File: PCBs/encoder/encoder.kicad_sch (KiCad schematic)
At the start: 16 parts, among them J1 Conn_01x04, J2 Conn_01x04, J3 Conn_01x04, U1 AS5600-ASOT, U2 STM32G031G6Ux

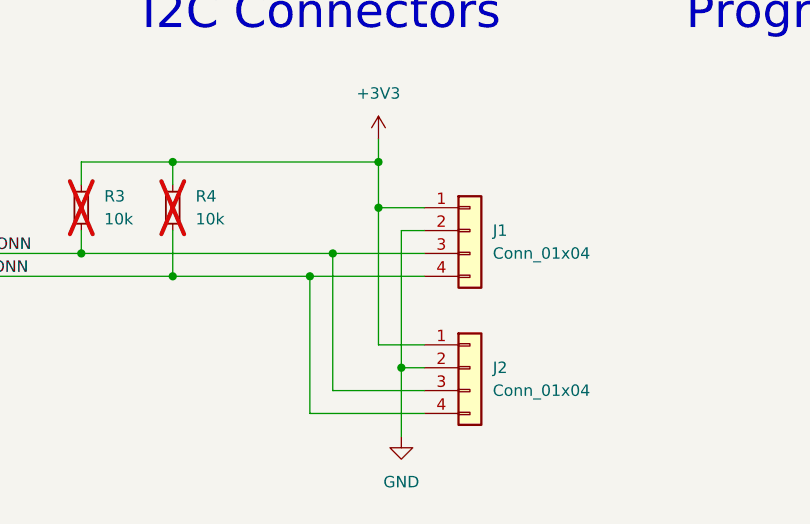
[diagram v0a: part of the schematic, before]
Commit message: fix encoder board fuck you ben
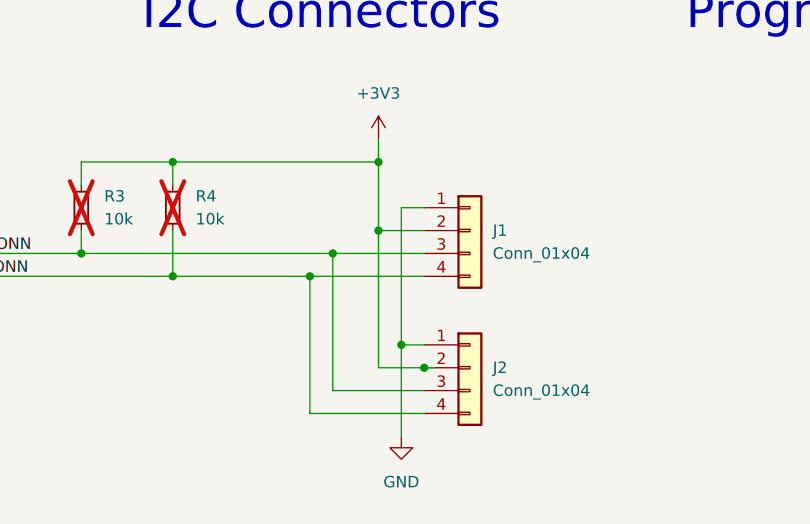
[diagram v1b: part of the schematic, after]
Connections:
- net +3V3: now also J1.2 (Pin_2), J2.2 (Pin_2); no longer J1.1 (Pin_1), J2.1 (Pin_1)
- net GND: now also J1.1 (Pin_1), J2.1 (Pin_1); no longer J1.2 (Pin_2), J2.2 (Pin_2)
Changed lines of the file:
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@@
+	)
+	(junction
+		(at 167.64 152.4)
+		(diameter 0)
+		(color 0 0 0 0)
 	)
 	(junction
@@
 	)
 	(junction
+		(at 162.56 137.16)
+		(diameter 0)
+		(color 0 0 0 0)
+	)
+	(junction
 		(at 139.7 129.54)
 		(diameter 0)
@@
 	)
 	(junction
-		(at 162.56 134.62)
-		(diameter 0)
-		(color 0 0 0 0)
-	)
-	(junction
-		(at 165.1 152.4)
-		(diameter 0)
-		(color 0 0 0 0)
-	)
-	(junction
 		(at 162.56 129.54)
 		(diameter 0)
@@
 	)
 	(junction
+		(at 165.1 149.86)
+		(diameter 0)
+		(color 0 0 0 0)
+	)
+	(junction
 		(at 226.06 53.34)
 		(diameter 0)
@@
 	(wire
 		(pts
+			(xy 162.56 152.4) (xy 167.64 152.4)
+		)
+		(stroke
+			(width 0)
+			(type default)
+		)
+	)
+	(wire
+		(pts
 			(xy 129.54 139.7) (xy 157.48 139.7)
 		)
@@
 	(wire
 		(pts
-			(xy 162.56 134.62) (xy 167.64 134.62)
-		)
-		(stroke
-			(width 0)
-			(type default)
-		)
-	)
-	(wire
-		(pts
 			(xy 127 76.2) (xy 149.86 76.2)
 		)
@@
 	(wire
 		(pts
-			(xy 165.1 152.4) (xy 167.64 152.4)
+			(xy 165.1 134.62) (xy 167.64 134.62)
 		)
 		(stroke
@@
 	(wire
 		(pts
+			(xy 165.1 149.86) (xy 167.64 149.86)
+		)
+		(stroke
+			(width 0)
+			(type default)
+		)
+	)
+	(wire
+		(pts
+			(xy 162.56 137.16) (xy 167.64 137.16)
+		)
+		(stroke
+			(width 0)
+			(type default)
+		)
+	)
+	(wire
+		(pts
+			(xy 165.1 160.02) (xy 165.1 149.86)
+		)
+		(stroke
+			(width 0)
+			(type default)
+		)
+	)
+	(wire
+		(pts
 			(xy 116.84 60.96) (xy 116.84 63.5)
 		)
@@
 	(wire
 		(pts
+			(xy 165.1 149.86) (xy 165.1 134.62)
+		)
+		(stroke
+			(width 0)
+			(type default)
+		)
+	)
+	(wire
+		(pts
 			(xy 127 71.12) (xy 127 76.2)
 		)
@@
 	(wire
 		(pts
-			(xy 162.56 134.62) (xy 162.56 129.54)
-		)
-		(stroke
-			(width 0)
-			(type default)
-		)
-	)
-	(wire
-		(pts
 			(xy 109.22 78.74) (xy 109.22 81.28)
 		)
@@
 	(wire
 		(pts
+			(xy 167.64 152.4) (xy 168.91 152.4)
+		)
+		(stroke
+			(width 0)
+			(type default)
+		)
+	)
+	(wire
+		(pts
 			(xy 185.42 71.12) (xy 200.66 71.12)
 		)
@@
 	(wire
 		(pts
+			(xy 162.56 129.54) (xy 162.56 137.16)
+		)
+		(stroke
+			(width 0)
+			(type default)
+		)
+	)
+	(wire
+		(pts
 			(xy 226.06 50.8) (xy 226.06 53.34)
 		)
@@
 	(wire
 		(pts
+			(xy 162.56 137.16) (xy 162.56 152.4)
+		)
+		(stroke
+			(width 0)
+			(type default)
+		)
+	)
+	(wire
+		(pts
 			(xy 114.3 139.7) (xy 129.54 139.7)
 		)
@@
 	(wire
 		(pts
-			(xy 162.56 149.86) (xy 162.56 134.62)
-		)
-		(stroke
-			(width 0)
-			(type default)
-		)
-	)
-	(wire
-		(pts
 			(xy 116.84 63.5) (xy 127 63.5)
 		)
@@
 	(wire
 		(pts
-			(xy 167.64 149.86) (xy 162.56 149.86)
-		)
-		(stroke
-			(width 0)
-			(type default)
-		)
-	)
-	(wire
-		(pts
 			(xy 73.66 78.74) (xy 73.66 81.28)
 		)
@@
 	(wire
 		(pts
-			(xy 165.1 137.16) (xy 167.64 137.16)
-		)
-		(stroke
-			(width 0)
-			(type default)
-		)
-	)
-	(wire
-		(pts
 			(xy 185.42 68.58) (xy 200.66 68.58)
 		)
 		(stroke
-			(width 0)
-			(type default)
-		)
-	)
-	(wire
-		(pts
-			(xy 165.1 152.4) (xy 165.1 160.02)
-		)
-		(stroke
-			(width 0)
-			(type default)
-		)
-	)
-	(wire
-		(pts
-			(xy 165.1 137.16) (xy 165.1 152.4)
-		)
-		(stroke
